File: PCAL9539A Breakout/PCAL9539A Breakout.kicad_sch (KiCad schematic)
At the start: 2 parts

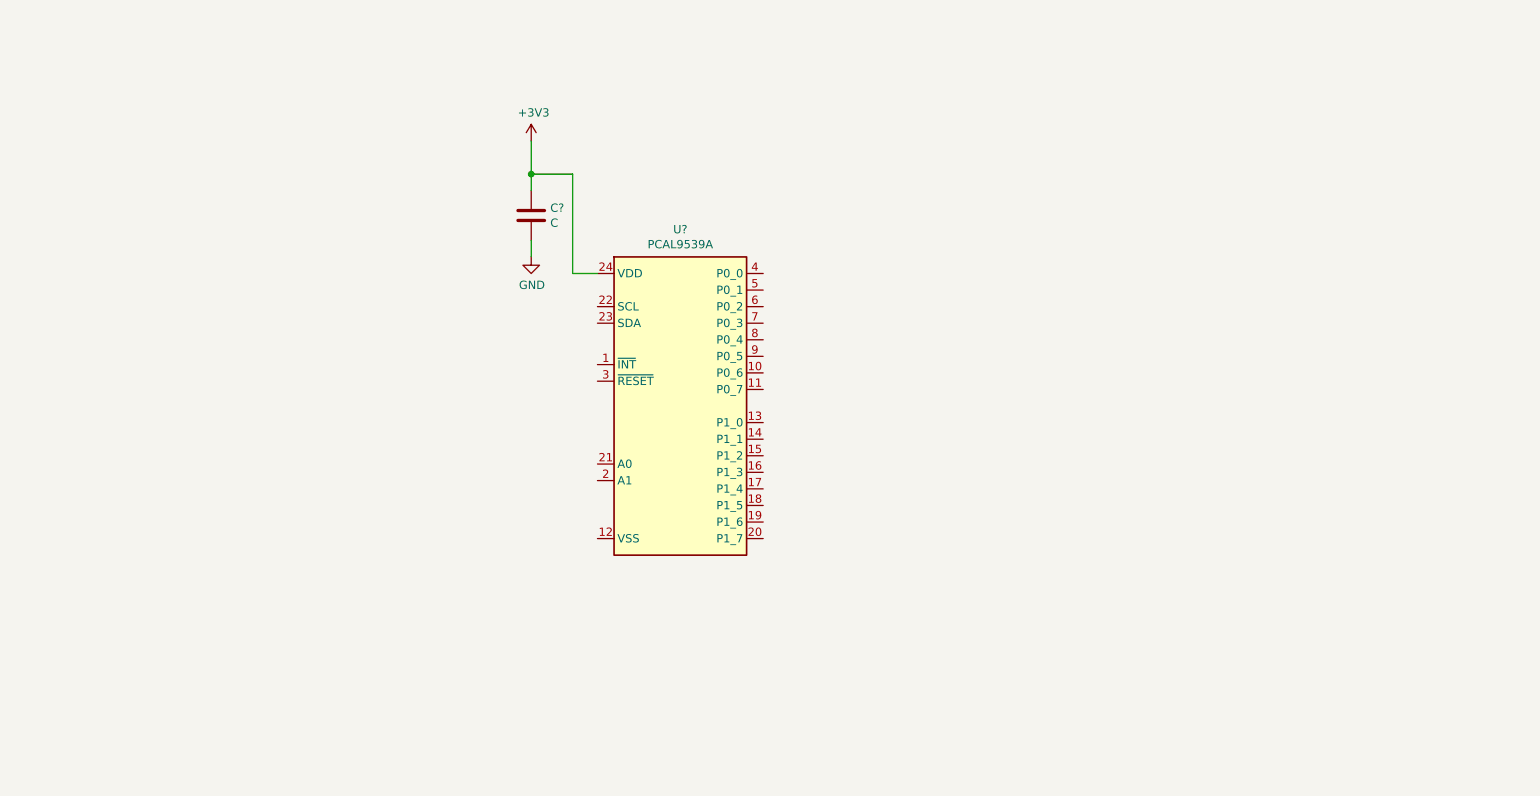
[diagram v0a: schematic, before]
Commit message: schematic, copper
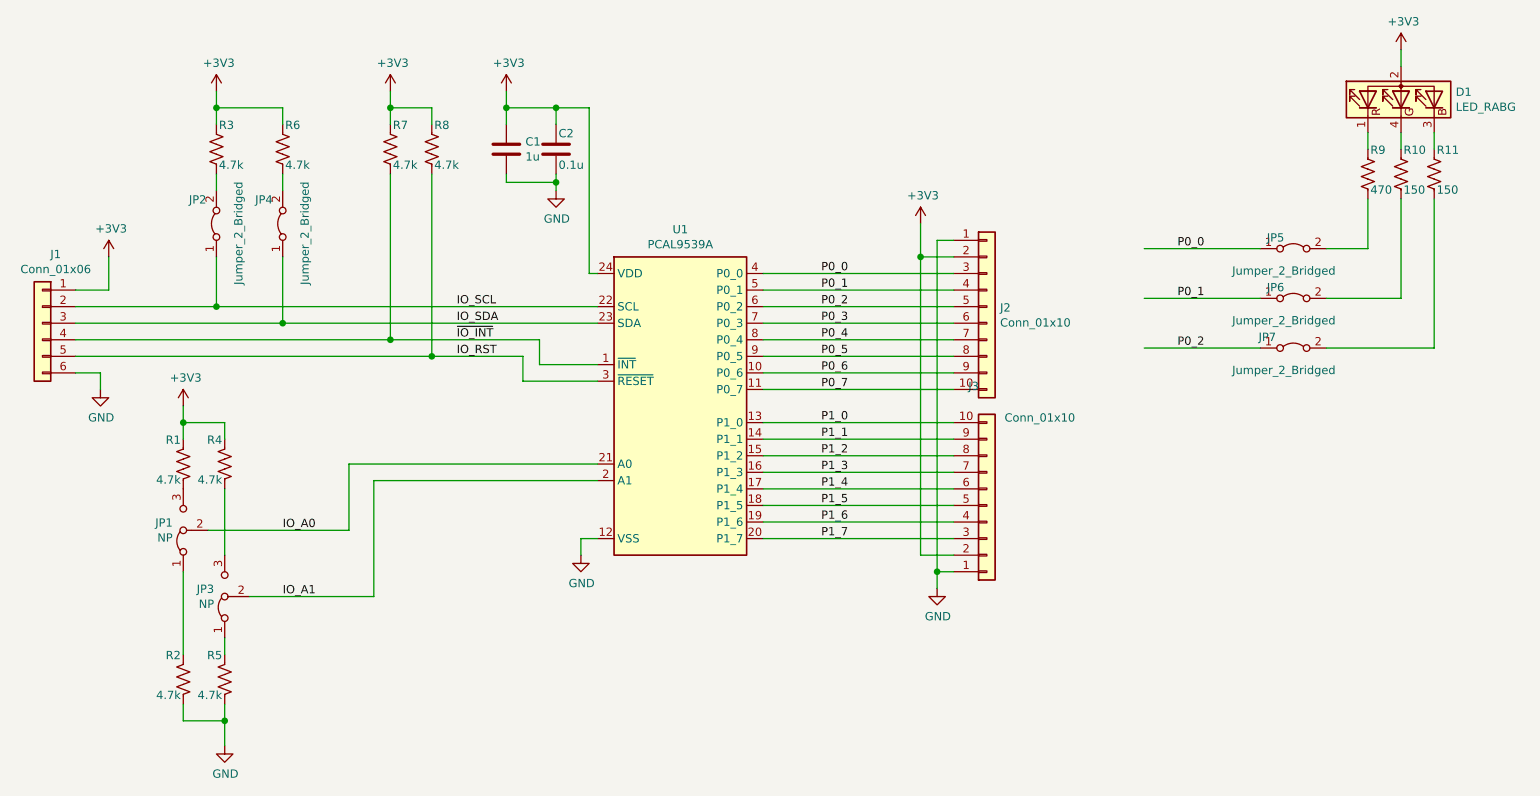
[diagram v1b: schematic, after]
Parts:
- added C1: 1u, Capacitor_SMD:C_0603_1608Metric, symbol Device:C
- added D1: LED_RABG, LED_SMD:LED_Kingbright_AAA3528ESGCT, symbol Device:LED_RABG
- added J1: Conn_01x06, Connector_PinHeader_2.54mm:PinHeader_1x06_P2.54mm_Vertical, symbol Connector_Generic:Conn_01x06
- added J2, J3: Conn_01x10, Connector_PinHeader_2.54mm:PinHeader_1x10_P2.54mm_Vertical, symbol Connector_Generic:Conn_01x10
- added JP1, JP3: NP, Connector_PinHeader_2.54mm:PinHeader_1x03_P2.54mm_Vertical, symbol Jumper:Jumper_3_Bridged12
- added JP2, JP4, JP5, JP6, JP7: Jumper_2_Bridged, Connector_PinHeader_2.54mm:PinHeader_1x02_P2.54mm_Vertical, symbol Jumper:Jumper_2_Bridged
- added R1, R2, R3, R4, R5, R6, R7, R8: 4.7k, Resistor_SMD:R_0603_1608Metric, symbol Device:R_US
- added R10, R11: 150, Resistor_SMD:R_0603_1608Metric, symbol Device:R_US
- added R9: 470, Resistor_SMD:R_0603_1608Metric, symbol Device:R_US
- C2: renamed from C?; value C -> 0.1u; footprint (none) -> Capacitor_SMD:C_0603_1608Metric
- gave numbers to parts that had none: 1
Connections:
- net +3V3: now also C1.1, D1.2 (A), J1.1 (Pin_1), J2.2 (Pin_2), J3.2 (Pin_2), R1.1, R3.1, R4.1, R6.1, R7.1, R8.1
- net GND: now also U1.12 (VSS), C1.2, J1.6 (Pin_6), J2.1 (Pin_1), J3.1 (Pin_1), R2.2, R5.2
- net ~IO_INT: now reaches U1.1 (~INT)
- net ~IO_INT: now also J1.4 (Pin_4), R7.2
- net P0_6: now reaches U1.10 (P0_6)
- net P0_6: now also J2.9 (Pin_9)
- net P0_7: now reaches U1.11 (P0_7)
- net P0_7: now also J2.10 (Pin_10)
- net P1_0: now reaches U1.13 (P1_0)
- net P1_0: now also J3.10 (Pin_10)
- net P1_1: now reaches U1.14 (P1_1)
- net P1_1: now also J3.9 (Pin_9)
- net P1_2: now reaches U1.15 (P1_2)
- net P1_2: now also J3.8 (Pin_8)
- net P1_3: now reaches U1.16 (P1_3)
- net P1_3: now also J3.7 (Pin_7)
- net P1_4: now reaches U1.17 (P1_4)
- net P1_4: now also J3.6 (Pin_6)
- net P1_5: now reaches U1.18 (P1_5)
- net P1_5: now also J3.5 (Pin_5)
- net P1_6: now reaches U1.19 (P1_6)
- net P1_6: now also J3.4 (Pin_4)
- net IO_A1: now reaches U1.2 (A1)
- net IO_A1: now also JP3.2 (C)
- net P1_7: now reaches U1.20 (P1_7)
- net P1_7: now also J3.3 (Pin_3)
- net IO_A0: now reaches U1.21 (A0)
- net IO_A0: now also JP1.2 (C)
- net IO_SCL: now reaches U1.22 (SCL)
- net IO_SCL: now also J1.2 (Pin_2), JP2.1 (A)
- net IO_SDA: now reaches U1.23 (SDA)
- net IO_SDA: now also J1.3 (Pin_3), JP4.1 (A)
- net IO_RST: now reaches U1.3 (~RESET)
- net IO_RST: now also J1.5 (Pin_5), R8.2
- net P0_0: now reaches U1.4 (P0_0)
- net P0_0: now also J2.3 (Pin_3), JP5.1 (A)
- net P0_1: now reaches U1.5 (P0_1)
- net P0_1: now also J2.4 (Pin_4), JP6.1 (A)
- net P0_2: now reaches U1.6 (P0_2)
- net P0_2: now also J2.5 (Pin_5), JP7.1 (A)
- net P0_3: now reaches U1.7 (P0_3)
- net P0_3: now also J2.6 (Pin_6)
- net P0_4: now reaches U1.8 (P0_4)
- net P0_4: now also J2.7 (Pin_7)
- net P0_5: now reaches U1.9 (P0_5)
- net P0_5: now also J2.8 (Pin_8)
- new net: D1.1 (RK), R9.1
- new net: JP5.2 (B), R9.2
- new net: JP3.1 (A), R5.1
- new net: JP2.2 (B), R3.2
- new net: JP1.3 (B), R1.2
- new net: JP1.1 (A), R2.1
- new net: JP3.3 (B), R4.2
- new net: D1.3 (BK), R11.1
- new net: D1.4 (GK), R10.1
- new net: JP4.2 (B), R6.2
- new net: JP7.2 (B), R11.2
- new net: JP6.2 (B), R10.2
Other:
- moved on the sheet: C2
